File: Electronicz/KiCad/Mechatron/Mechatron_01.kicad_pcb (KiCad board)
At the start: 2 copper layers, 130 x 125 mm, 58 parts, among them J1 Conn_01x15_Socket, J10 Servo_1, J11 Servo_2, J12 Servo_3, J13 V_ESP32, J14 GND_ESP32, J15 Motor_1, J16 Motor_2, J17 Motor_3, J18 Motor_4, J19 V_LED_2, J2 Front, J20 V_LED_1, J21 V_LED_top, J22 GND_LED_top, J23 GND_LED_2, J24 GND_LED_1, J25 SD-Card-Reader, J26 AUDIOAMP, J27 Speaker, J28 Conn_01x01_Pin, J29 Conn_01x01_Pin, J3 Left_Front, J30 SW, J4 Left_Back, J5 Back, J6 Right_Back, J7 Right_Front, J8 GND_Battery, J9 V_Battery_Switch, Q1 LR_LED_Sensors, Q2 LR_3, Q3 LR_2, Q4 LR_1, Q5 LED_top, Q6 LED_2, Q7 LED_1

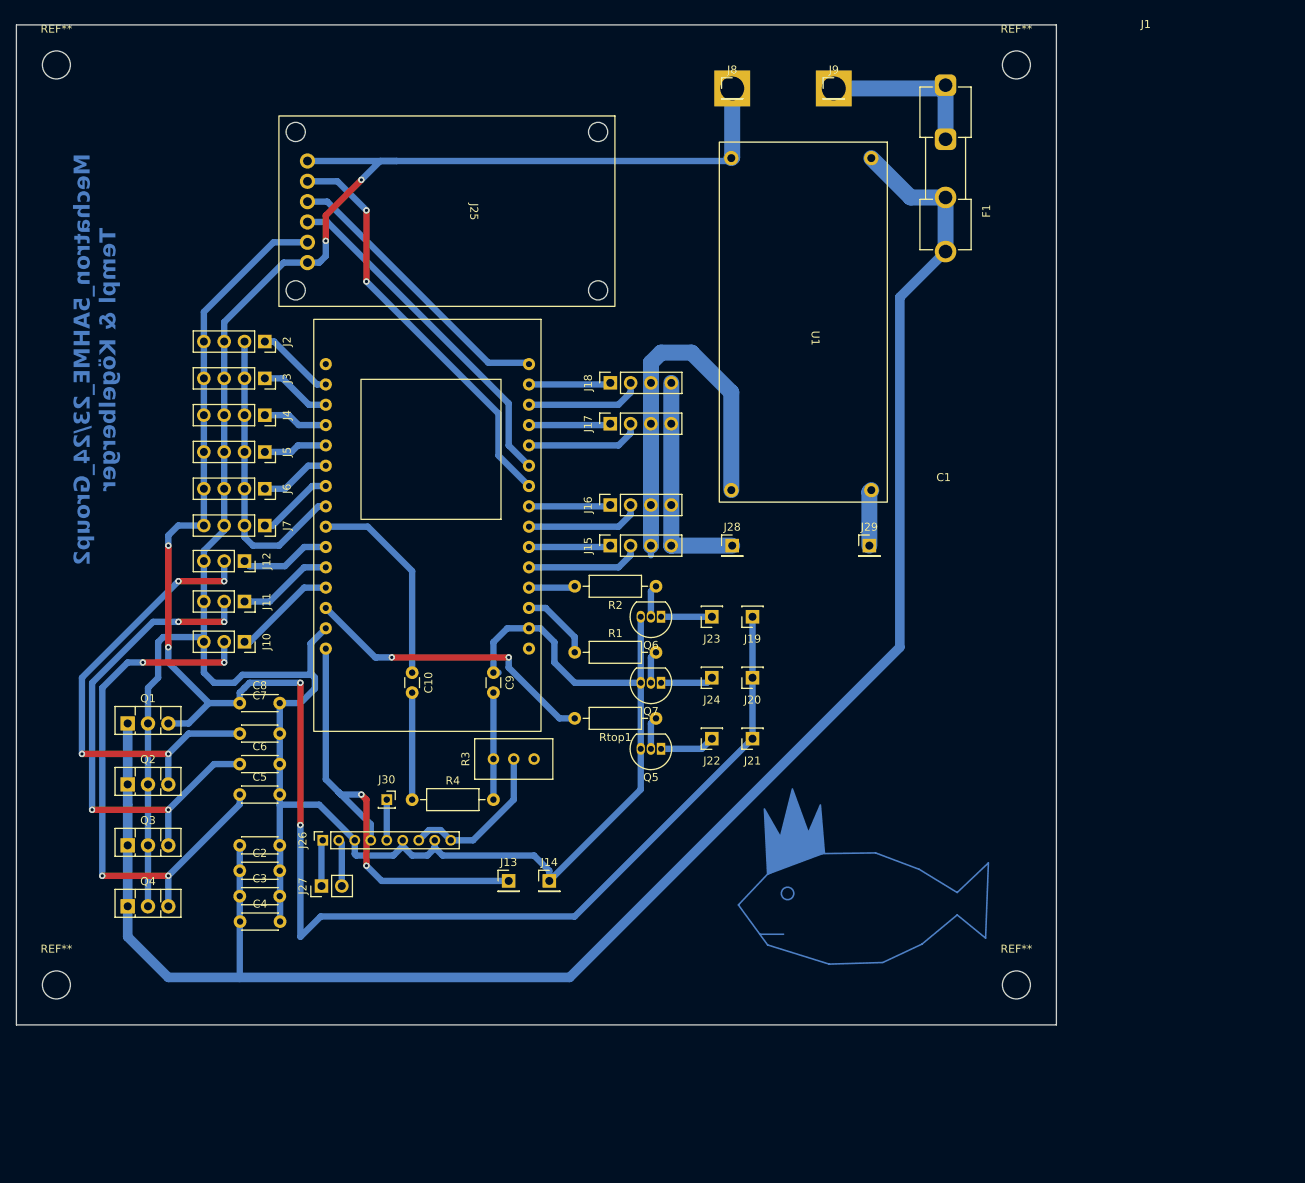
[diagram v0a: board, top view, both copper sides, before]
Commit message: export pcb and schematic pdfs
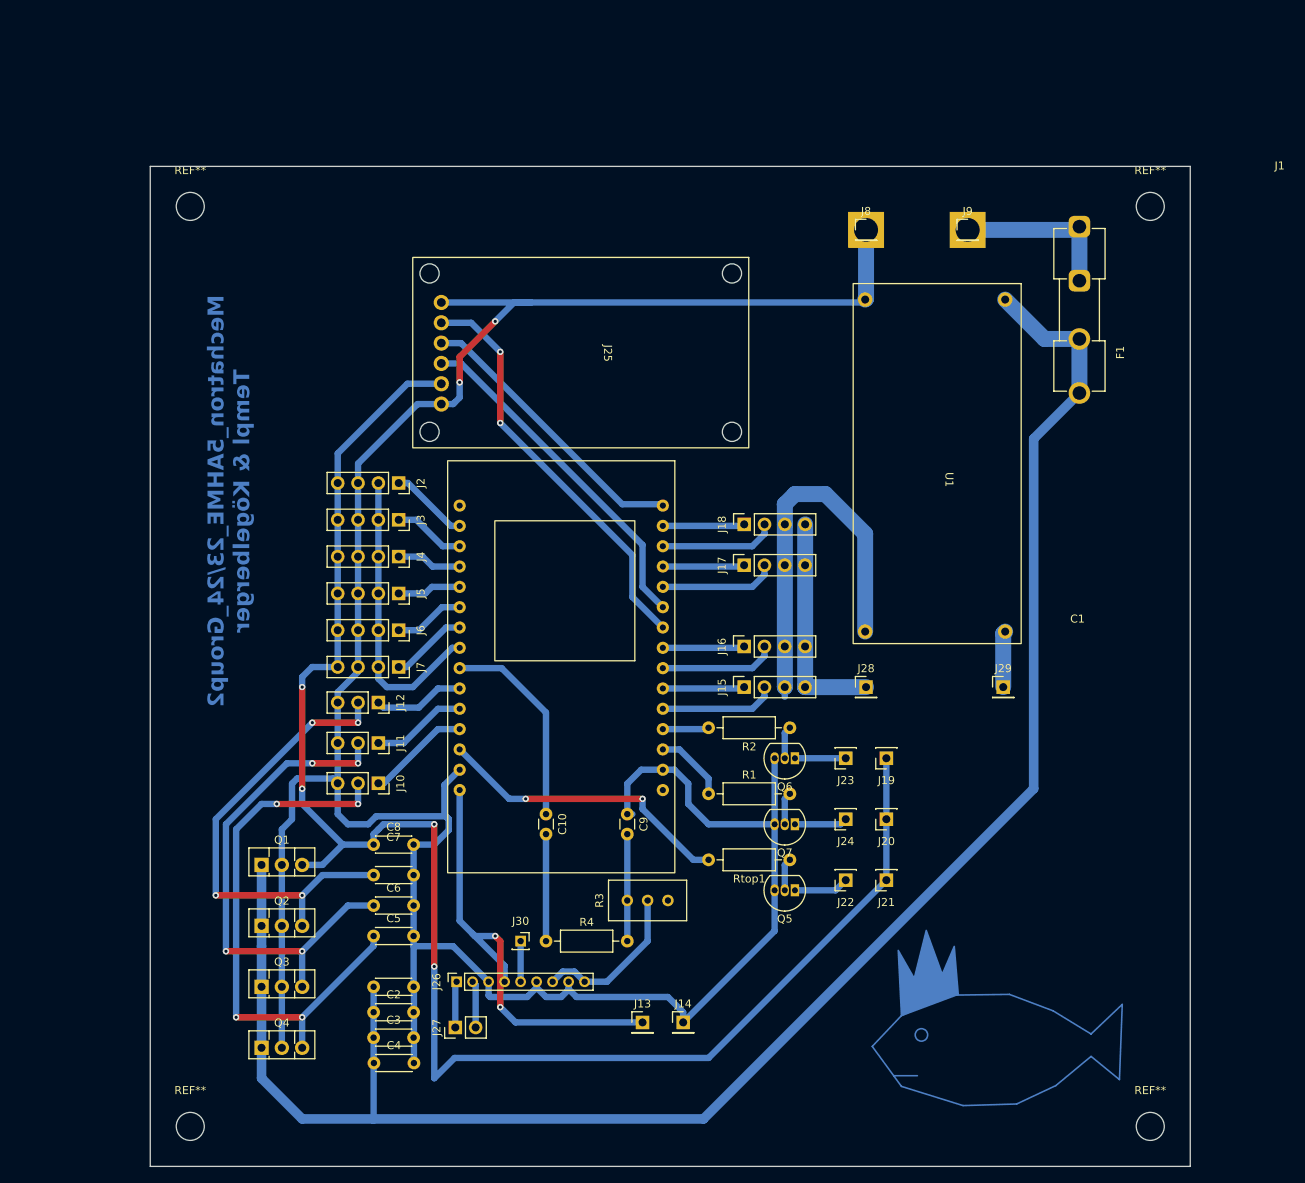
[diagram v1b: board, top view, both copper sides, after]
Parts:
- moved J20 24.3 mm to (128.7, 119.3)
- moved C5 24.3 mm to (64.7, 133.9)
- moved C6 24.3 mm to (64.7, 130.1)
- moved C7 24.3 mm to (64.7, 126.3)
- moved J17 24.3 mm to (111.0, 87.5)
- moved J19 24.3 mm to (128.7, 111.7)
- moved J21 24.3 mm to (128.7, 126.9)
- moved J24 24.3 mm to (123.7, 119.3)
- moved J25 24.3 mm to (111.5, 49.1)
- moved J26 24.3 mm to (75.0, 139.6)
- moved J6 24.3 mm to (67.8, 95.7)
- moved Q5 24.3 mm to (117.3, 128.2)
- moved J8 24.3 mm to (126.2, 45.6)
- moved J9 24.3 mm to (138.9, 45.6)
- moved U1 24.3 mm to (143.6, 54.3)
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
